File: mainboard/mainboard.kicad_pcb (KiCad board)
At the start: 2 copper layers, 100 x 100 mm, 7 parts, among them Q1 PMV32UP, U1 ESP32-WROOM-32, U2 tps63070, U3 tps63070, U4 tps63070, U5 CP2102N-A01-GQFN24

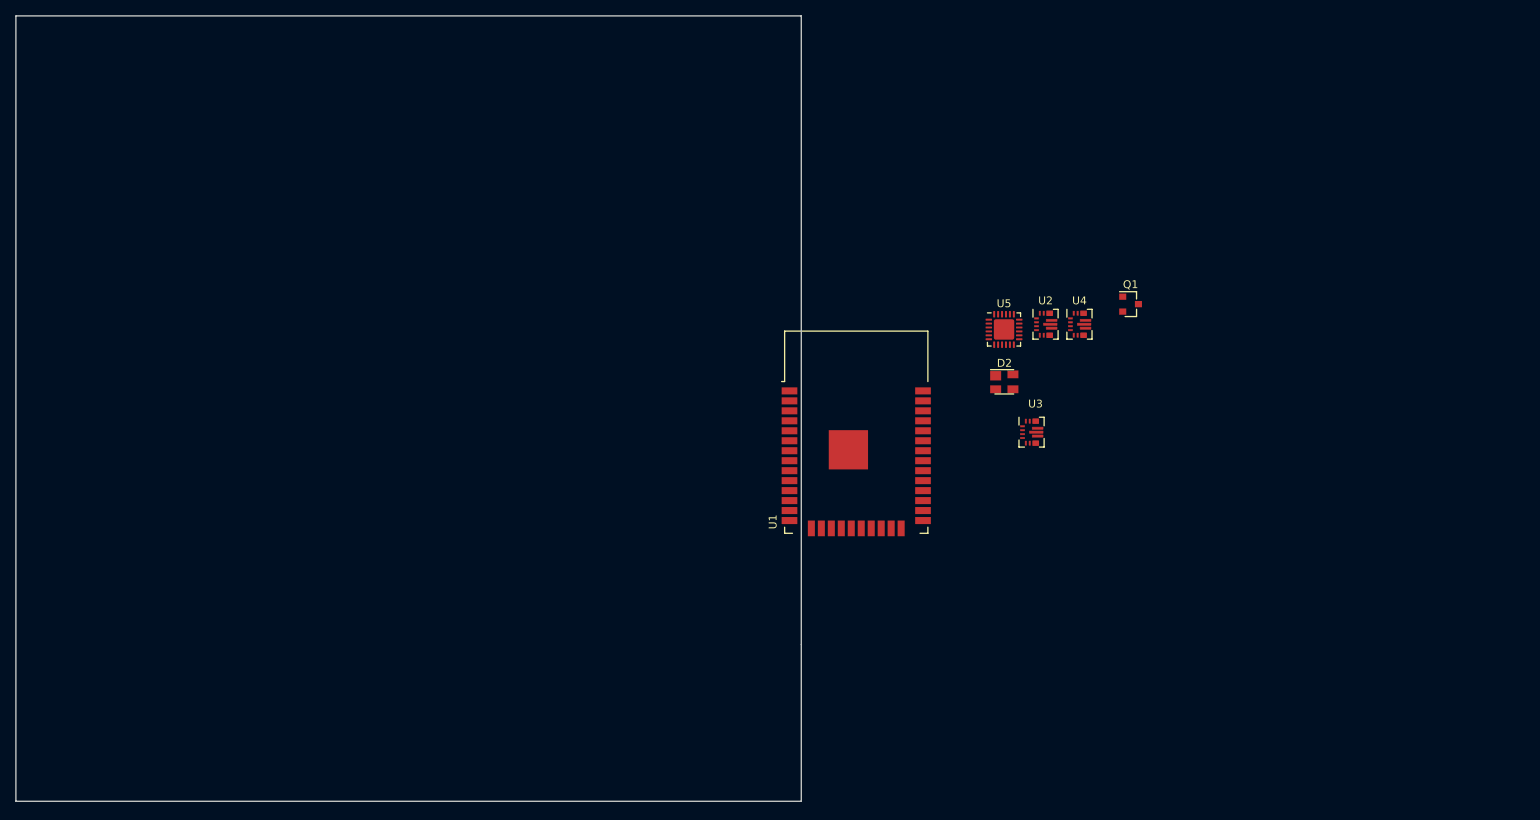
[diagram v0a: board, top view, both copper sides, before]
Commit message: Layouting WIP
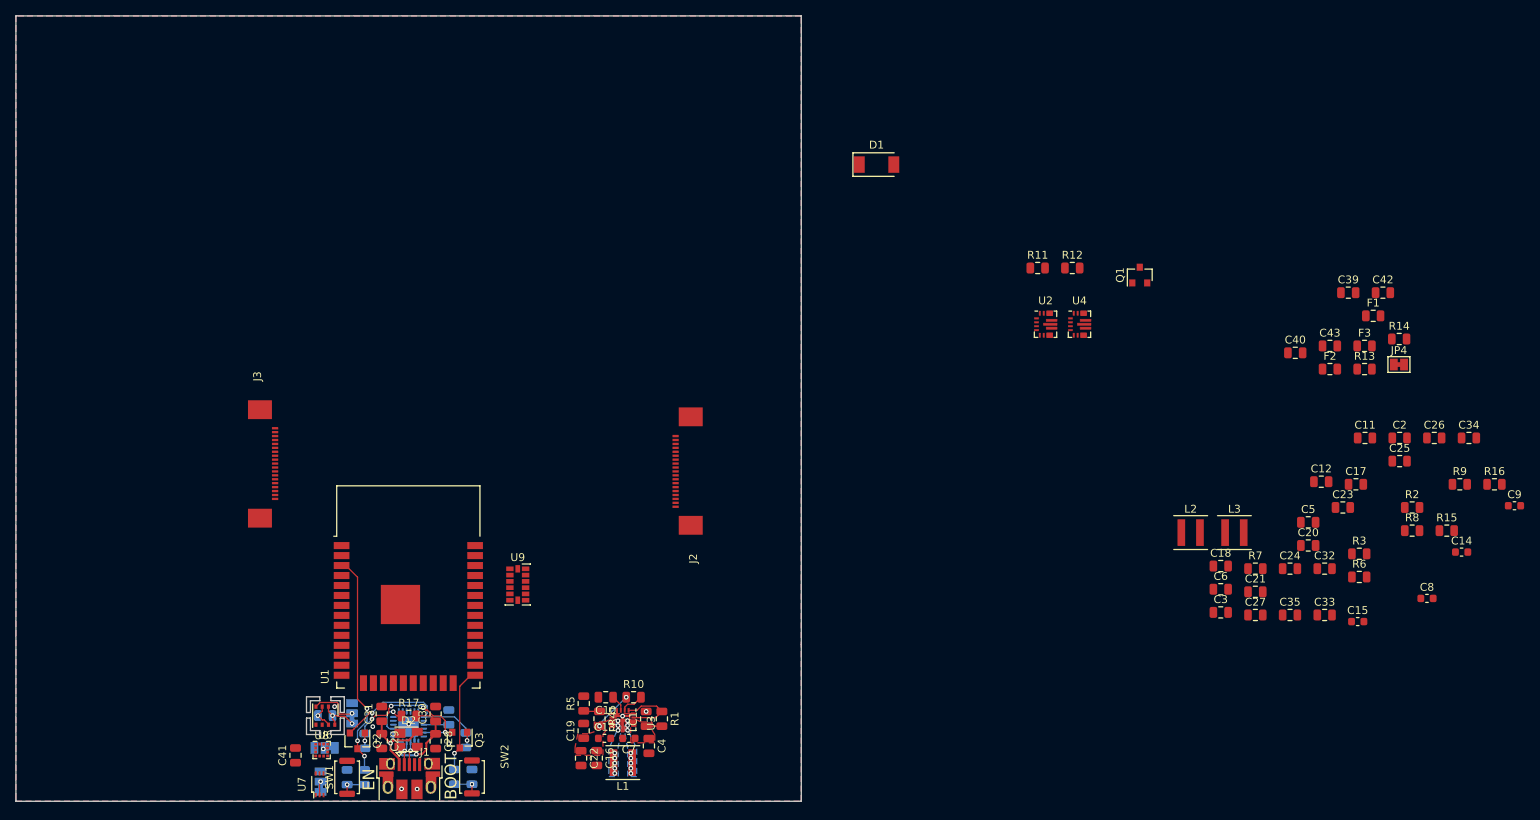
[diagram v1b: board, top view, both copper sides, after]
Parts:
- added C1: C, Capacitor_SMD:C_0805_2012Metric, F.Cu at (110.2, 119.5)
- added C10: 100 nC, Capacitor_SMD:C_0805_2012Metric, F.Cu at (105.1, 116.8)
- added C11: 100 nC, Capacitor_SMD:C_0805_2012Metric, F.Cu at (201.8, 83.7)
- added C12: 100 nC, Capacitor_SMD:C_0805_2012Metric, F.Cu at (196.2, 89.3)
- added C13: C, Capacitor_SMD:C_0603_1608Metric, F.Cu at (105.0, 122.0)
- added C14: C, Capacitor_SMD:C_0603_1608Metric, F.Cu at (214.1, 98.3)
- added C15: C, Capacitor_SMD:C_0603_1608Metric, F.Cu at (200.8, 107.1)
- added C16: C, Capacitor_SMD:C_0805_2012Metric, F.Cu at (104.0, 124.5)
- added C17: C, Capacitor_SMD:C_0805_2012Metric, F.Cu at (200.6, 89.6)
- added C18: C, Capacitor_SMD:C_0805_2012Metric, F.Cu at (183.4, 100.0)
- added C19: C, Capacitor_SMD:C_0805_2012Metric, F.Cu at (102.3, 121.0)
- added C2: C, Capacitor_SMD:C_0805_2012Metric, F.Cu at (206.2, 83.7)
- added C20: C, Capacitor_SMD:C_0805_2012Metric, F.Cu at (194.6, 97.4)
- added C21: C, Capacitor_SMD:C_0805_2012Metric, F.Cu at (187.8, 103.3)
- added C22: C, Capacitor_SMD:C_0805_2012Metric, F.Cu at (102.0, 124.5)
- added C23: C, Capacitor_SMD:C_0805_2012Metric, F.Cu at (199.0, 92.6)
- added C24: C, Capacitor_SMD:C_0805_2012Metric, F.Cu at (192.2, 100.4)
- added C25: C, Capacitor_SMD:C_0805_2012Metric, F.Cu at (206.2, 86.7)
- added C26: C, Capacitor_SMD:C_0805_2012Metric, F.Cu at (210.6, 83.7)
- added C27: C, Capacitor_SMD:C_0805_2012Metric, F.Cu at (187.8, 106.3)
- added C28: C, Capacitor_SMD:C_0805_2012Metric, F.Cu at (83.4, 122.3)
- added C29: C, Capacitor_SMD:C_0805_2012Metric, F.Cu at (76.6, 122.3)
- added C3: C, Capacitor_SMD:C_0805_2012Metric, F.Cu at (183.4, 106.0)
- added C30: C, Capacitor_SMD:C_0805_2012Metric, F.Cu at (83.4, 118.9)
- added C31: C, Capacitor_SMD:C_0805_2012Metric, F.Cu at (76.6, 118.9)
- added C32: C, Capacitor_SMD:C_0805_2012Metric, F.Cu at (196.6, 100.4)
- added C33: C, Capacitor_SMD:C_0805_2012Metric, F.Cu at (196.6, 106.3)
- added C34: C, Capacitor_SMD:C_0805_2012Metric, F.Cu at (215.0, 83.7)
- added C35: C, Capacitor_SMD:C_0805_2012Metric, F.Cu at (192.2, 106.3)
- added C36: 1 nC, Capacitor_SMD:C_0805_2012Metric, B.Cu at (72.2, 126.9)
- added C37: 1 nC, Capacitor_SMD:C_0805_2012Metric, B.Cu at (88.1, 126.9)
- added C38: 100 nC, Capacitor_SMD:C_0805_2012Metric, B.Cu at (69.4, 119.1)
- added C39: 1 uC, Capacitor_SMD:C_0805_2012Metric, F.Cu at (199.7, 65.2)
- added C4: C, Capacitor_SMD:C_0805_2012Metric, F.Cu at (110.6, 123.0)
- added C40: 100 nC, Capacitor_SMD:C_0805_2012Metric, F.Cu at (192.9, 72.9)
- added C41: 100 nC, Capacitor_SMD:C_0805_2012Metric, F.Cu at (65.6, 124.2)
- added C42: 100 nC, Capacitor_SMD:C_0805_2012Metric, F.Cu at (204.1, 65.2)
- added C43: 100 nC, Capacitor_SMD:C_0805_2012Metric, F.Cu at (197.3, 72.0)
- added C5: C, Capacitor_SMD:C_0805_2012Metric, F.Cu at (194.6, 94.5)
- added C6: C, Capacitor_SMD:C_0805_2012Metric, F.Cu at (183.4, 103.0)
- added C7: C, Capacitor_SMD:C_0603_1608Metric, F.Cu at (108.0, 122.0)
- added C8: C, Capacitor_SMD:C_0603_1608Metric, F.Cu at (209.7, 104.2)
- added C9: C, Capacitor_SMD:C_0603_1608Metric, F.Cu at (220.8, 92.4)
- added D1: PMEG3050EP,115, mainboard:SOD-128-2, F.Cu at (139.6, 48.9)
- added F1: Fuse, Fuse:Fuse_0805_2012Metric, F.Cu at (202.8, 68.2)
- added F2: Fuse, Fuse:Fuse_0805_2012Metric, F.Cu at (197.3, 75.0)
- added F3: Fuse, Fuse:Fuse_0805_2012Metric, F.Cu at (201.7, 72.0)
- added J1: USB_B_Micro, Connector_USB:USB_Micro-B_Amphenol_10103594-0001LF_Horizontal, F.Cu at (80.1, 127.1)
- added J2: Conn_01x19_MountingPin, mainboard:Molex_Easy-On_52746-1971_1x19_P0.5mm_Horizontal, F.Cu at (114.0, 88.0)
- added J3: Conn_01x19_MountingPin, mainboard:Molex_Easy-On_52746-1971_1x19_P0.5mm_Horizontal, F.Cu at (63.0, 87.0)
- added JP1: Jumper_3_Bridged12, Jumper:SolderJumper-3_P1.3mm_Bridged12_Pad1.0x1.5mm, B.Cu at (68.8, 127.5)
- added JP2: Jumper_3_Bridged12, Jumper:SolderJumper-3_P1.3mm_Bridged12_Pad1.0x1.5mm, B.Cu at (72.8, 118.8)
- added JP3: Jumper_3_Bridged12, Jumper:SolderJumper-3_P1.3mm_Bridged12_Pad1.0x1.5mm, B.Cu at (69.3, 123.2)
- added JP4: Jumper, Jumper:SolderJumper-2_P1.3mm_Bridged_Pad1.0x1.5mm, F.Cu at (206.1, 74.4)
- added L1: L, Inductor_SMD:L_Coilcraft_XxL4020, F.Cu at (107.3, 125.1)
- added L2: L, Inductor_SMD:L_Coilcraft_XxL4020, F.Cu at (179.6, 95.8)
- added L3: L, Inductor_SMD:L_Coilcraft_XxL4020, F.Cu at (185.2, 95.8)
- added Q2: MMBT3904, Package_TO_SOT_SMD:SOT-23, F.Cu at (73.5, 122.3)
- added Q3: MMBT3904, Package_TO_SOT_SMD:SOT-23, F.Cu at (86.5, 122.2)
- added R1: 10 kR, Resistor_SMD:R_0805_2012Metric, F.Cu at (112.2, 119.5)
- added R10: 10 kR, Resistor_SMD:R_0805_2012Metric, F.Cu at (108.7, 116.8)
- added R11: 10 kR, Resistor_SMD:R_0805_2012Metric, F.Cu at (160.1, 62.1)
- added R12: 10 kR, Resistor_SMD:R_0805_2012Metric, F.Cu at (164.5, 62.1)
- added R13: 2.2 kR, Resistor_SMD:R_0805_2012Metric, F.Cu at (201.7, 75.0)
- added R14: 2.2 kR, Resistor_SMD:R_0805_2012Metric, F.Cu at (206.1, 71.1)
- added R15: 100 kR, Resistor_SMD:R_0805_2012Metric, F.Cu at (212.2, 95.5)
- added R16: 1 kR, Resistor_SMD:R_0805_2012Metric, F.Cu at (218.3, 89.6)
- added R17: 4.7 kR, Resistor_SMD:R_0805_2012Metric, F.Cu at (80.0, 119.1)
- added R18: 470 R, Resistor_SMD:R_0805_2012Metric, B.Cu at (85.1, 119.3)
- added R19: 12 kR, Resistor_SMD:R_0805_2012Metric, B.Cu at (74.4, 122.3)
- added R2: 10 kR, Resistor_SMD:R_0805_2012Metric, F.Cu at (207.8, 92.6)
- added R20: 12 kR, Resistor_SMD:R_0805_2012Metric, B.Cu at (87.3, 122.2)
- added R21: 470 R, Resistor_SMD:R_0805_2012Metric, B.Cu at (74.4, 126.9)
- added R22: 470 R, Resistor_SMD:R_0805_2012Metric, B.Cu at (85.8, 126.9)
- added R3: 10 kR, Resistor_SMD:R_0805_2012Metric, F.Cu at (201.1, 98.5)
- added R4: 470 kR, Resistor_SMD:R_0805_2012Metric, F.Cu at (104.3, 119.5)
- added R5: 150 kR, Resistor_SMD:R_0805_2012Metric, F.Cu at (102.3, 117.5)
- added R6: 470 kR, Resistor_SMD:R_0805_2012Metric, F.Cu at (201.1, 101.4)
- added R7: 120 kR, Resistor_SMD:R_0805_2012Metric, F.Cu at (187.8, 100.4)
- added R8: 470 kR, Resistor_SMD:R_0805_2012Metric, F.Cu at (207.8, 95.5)
- added R9: 120 kR, Resistor_SMD:R_0805_2012Metric, F.Cu at (213.8, 89.6)
- added SW1: SW_Push, Button_Switch_SMD:SW_Push_SPST_NO_Alps_SKRK, F.Cu at (72.2, 127.0)
- added SW2: SW_Push, Button_Switch_SMD:SW_Push_SPST_NO_Alps_SKRK, F.Cu at (88.1, 126.9)
- added U6: BME680, Package_LGA:Bosch_LGA-8_3x3mm_P0.8mm_ClockwisePinNumbering, F.Cu at (69.4, 119.1)
- added U7: BH1750FVI, mainboard:WSOF6I, F.Cu at (68.7, 127.8)
- added U8: LIS3MDL, Package_LGA:LGA-12_2x2mm_P0.5mm, F.Cu at (68.9, 123.5)
- added U9: ADXL343, Package_LGA:LGA-14_3x5mm_P0.8mm_LayoutBorder1x6y, F.Cu at (93.9, 102.4)
- Q1: value PMV32UP -> DMG2301L
- U5: moved to B.Cu
- moved U5 91.1 mm to (80.0, 120.5), turned to 90 degrees
- moved D2 88.5 mm to (80.0, 122.1)
- moved U3 63.6 mm to (107.3, 119.6), turned to 270 degrees
- moved U1 60.3 mm to (80.0, 105.7)
- moved Q1 3.88 mm to (173.1, 63.0), turned to 90 degrees
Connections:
- Q1 pad 3: VDC -> Net-(F3-Pad1)
- U1 pad 10: Net-(U1-Pad10) -> /SCL
- U1 pad 11: Net-(U1-Pad11) -> /SDA
- U1 pad 12: Net-(U1-Pad12) -> /VCC1_EN
- U1 pad 14: /SOUT1 -> Net-(JP4-Pad1)
- U1 pad 27: Net-(U1-Pad27) -> /PG_VCC0
- U1 pad 28: Net-(U1-Pad28) -> /PG_VCC1
- U1 pad 30: Net-(U1-Pad30) -> /SCK
- U1 pad 31: Net-(U1-Pad31) -> /MISO
- U1 pad 33: Net-(U1-Pad33) -> /~CS_ACCEL
- U1 pad 36: Net-(U1-Pad36) -> /VCC0_EN
- U1 pad 37: Net-(U1-Pad37) -> /MOSI
- U1 pad 4: Net-(U1-Pad4) -> /DRDY
- U1 pad 5: Net-(U1-Pad5) -> /INT
- U1 pad 6: Net-(U1-Pad6) -> /INT1
- U1 pad 7: Net-(U1-Pad7) -> /INT2
- U2 pad 12: VBUS -> VDC
- U2 pad 14: /VCC_EN -> /VCC0_EN
- U2 pad 2: /~PG_VCC0 -> /PG_VCC0
- U2 pad 9: (no net) -> Net-(L2-Pad2)
- U3 pad 2: /~PG_3V3 -> /PG_3V3
- U3 pad 9: (no net) -> Net-(L1-Pad2)
- U4 pad 12: VBUS -> VDC
- U4 pad 14: /VCC_EN -> /VCC1_EN
- U4 pad 2: /~PG_VCC1 -> /PG_VCC1
- U4 pad 9: (no net) -> Net-(L3-Pad2)
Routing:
- net /EN: track 0.00 -> 28.6 mm, vias 0 -> 3
- net /RTS: track 0.00 -> 19.7 mm, vias 0 -> 1
- net /DTR: track 0.00 -> 18.5 mm, vias 0 -> 4
- net /IO0: track 0.00 -> 13.4 mm, vias 0 -> 1
- net Net-(C28-Pad1): track 0.00 -> 12.6 mm, vias 0 -> 1
- net VUSB: track 0.00 -> 12.1 mm, vias 0 -> 1
- net GND: track 0.00 -> 11.6 mm, vias 0 -> 9
- net Net-(R1-Pad1): track 0.00 -> 8.64 mm
- net +3V3: track 0.00 -> 8.36 mm, vias 0 -> 4
- net Net-(JP2-Pad2): track 0.00 -> 6.41 mm, vias 0 -> 1
- net Net-(R17-Pad1): track 0.00 -> 4.67 mm, vias 0 -> 1
- net Net-(R4-Pad1): track 0.00 -> 4.03 mm
- net /D+: track 0.00 -> 4.02 mm, vias 0 -> 1
- net /D-: track 0.00 -> 3.85 mm, vias 0 -> 1
- net Net-(C37-Pad2): track 0.00 -> 3.40 mm, vias 0 -> 1
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- added copper zone on F.Cu, net +3V3
- added copper zone on B.Cu, net GND
- added copper zone on F.Cu, net GND
- added copper zone on B.Cu, net Net-(L1-Pad1)
- added copper zone on B.Cu, net Net-(L1-Pad2)
- added copper zone on F.Cu, net VBUS
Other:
- outline, holes or cut-outs redrawn
- board text added: "BOOT"
- board text added: "EN"

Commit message: WIP
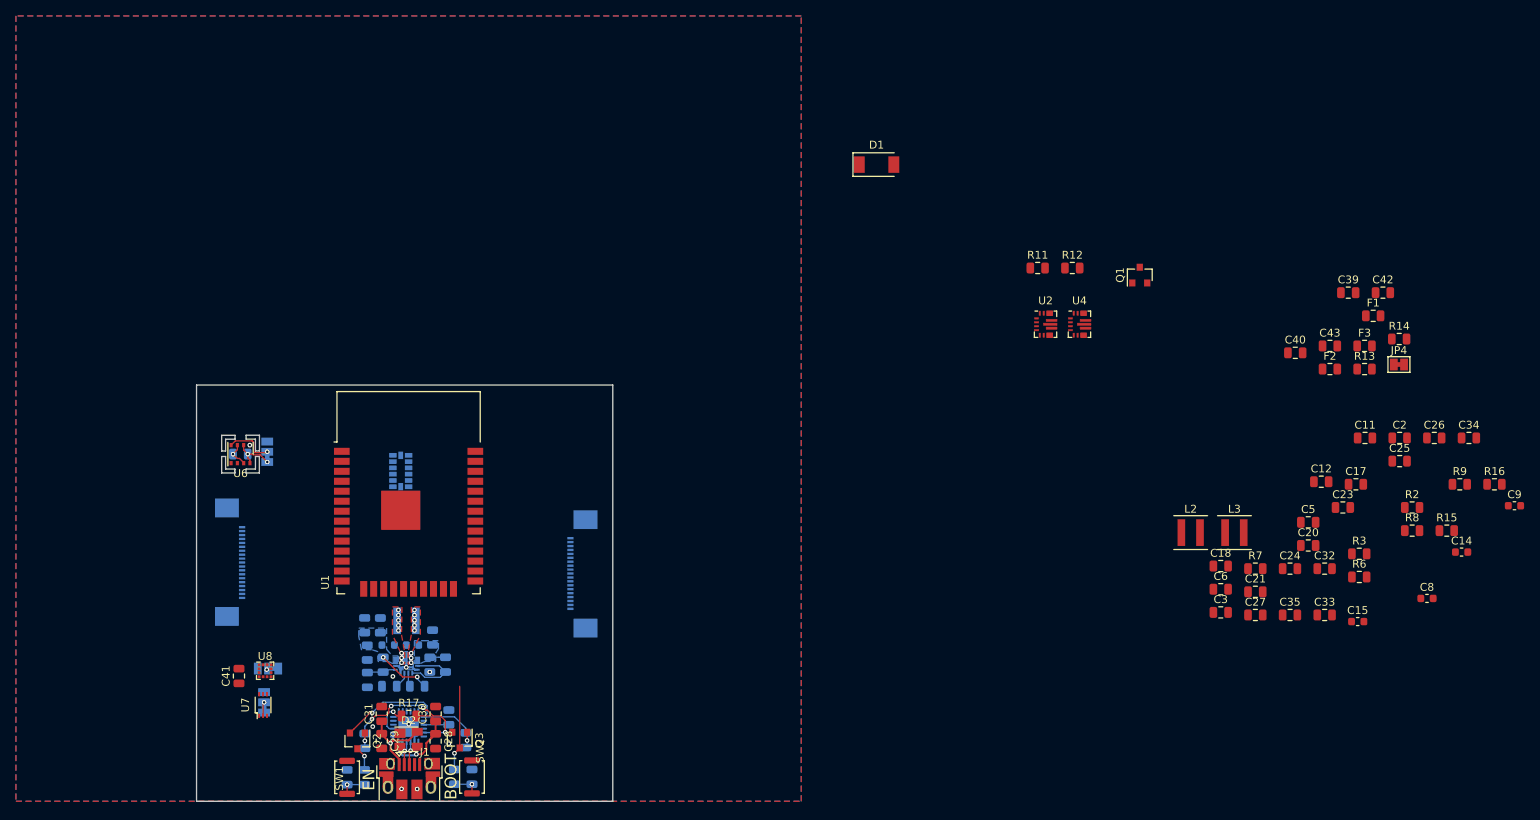
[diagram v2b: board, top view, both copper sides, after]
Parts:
- C1, C10, C13, C16, C19, C22, C4, C7, J2, J3, L1, R1, R10, R4, R5, U3, U9: moved to B.Cu
- moved U6 35.0 mm to (58.6, 85.8)
- moved C38 35.0 mm to (58.6, 85.8)
- moved JP2 35.0 mm to (62.0, 85.5)
- moved L1 32.9 mm to (79.7, 107.0)
- moved C22 32.3 mm to (74.4, 107.6), turned to 90 degrees
- moved C16 32.3 mm to (76.4, 107.6), turned to 90 degrees
- moved C4 30.8 mm to (83.0, 109.2), turned to 90 degrees
- moved C13 30.0 mm to (77.4, 110.1)
- moved C7 30.0 mm to (80.5, 110.1)
- moved C19 29.3 mm to (74.7, 111.1), turned to 270 degrees
- moved U3 28.4 mm to (79.7, 112.5), turned to 90 degrees
- moved C1 28.4 mm to (82.7, 112.6), turned to 270 degrees
- moved R1 28.4 mm to (84.7, 112.6), turned to 90 degrees
- moved R4 28.4 mm to (76.8, 112.6), turned to 90 degrees
- moved R5 27.7 mm to (74.8, 114.5), turned to 270 degrees
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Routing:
- net /EN: track 28.6 -> 3.07 mm, vias 3 -> 1
- net /IO0: track 13.4 -> 10.9 mm
- net +3V3: track 8.36 -> 10.5 mm
- net /PG_3V3: track 2.99 -> 1.75 mm
- net GND: vias 9 -> 10
- added copper zone on B.Cu, net +3V3
- added copper zone on F.Cu, net Net-(L1-Pad1)
- added copper zone on F.Cu, net Net-(L1-Pad2)
- added copper zone on B.Cu, net VBUS
- removed copper zone on F.Cu, net +3V3
- removed copper zone on B.Cu, net Net-(L1-Pad1)
- removed copper zone on B.Cu, net Net-(L1-Pad2)
- removed copper zone on F.Cu, net VBUS
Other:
- board size 100 x 100 mm -> 53 x 53 mm
